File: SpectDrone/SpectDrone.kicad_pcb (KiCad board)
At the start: 2 copper layers, 220.1 x 71.1 mm, 64 parts, among them J1 Camera, J2 GPS, J4 BME280, J5-1 BNO055-1, J5-2 BNO055-2, Q1 FDN340P, Q2 FDN340P, SW1 SW_Push, SW2 SW_Push, SW3 SW_Push, SW4 SW_Push, SW5 SW_Push, SW6 SW_Push, U1 C12666MA, U2 C12666MA, U3 LM7805_TO220, U4 MCP112-300E/TO, U5 MCP112-300E/TO, U6 LM7805_TO220, U7 Teensy3.2

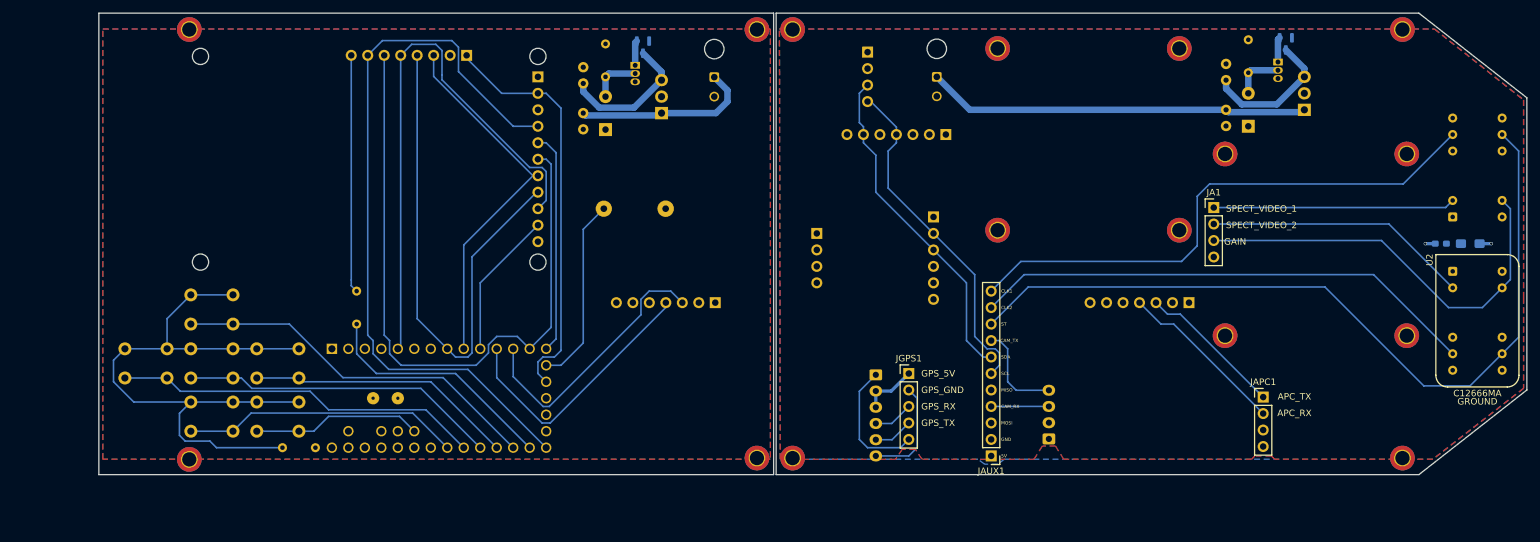
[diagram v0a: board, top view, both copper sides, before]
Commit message: SpectDrone Development
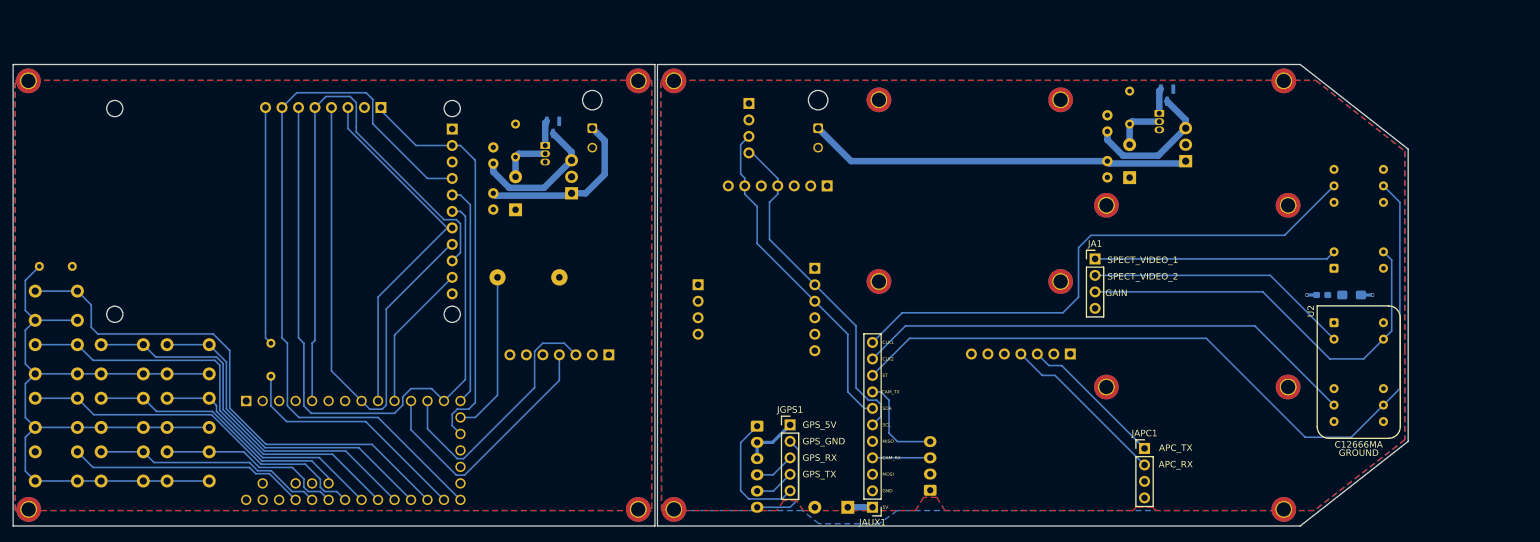
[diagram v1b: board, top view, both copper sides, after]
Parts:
- added D3: Ge, Diode_THT:D_T-1_P5.08mm_Horizontal, B.Cu at (170.9, 142.5)
- added SW0: SW_Push, Button_Switch_THT:SW_PUSH_6mm_H4.3mm, B.Cu at (52.2, 109.2)
- added SW7: SW_Push, Button_Switch_THT:SW_PUSH_6mm_H4.3mm, B.Cu at (72.5, 134.0)
- added SW8: SW_Push, Button_Switch_THT:SW_PUSH_6mm_H4.3mm, B.Cu at (62.4, 134.0)
- added SW9: SW_Push, Button_Switch_THT:SW_PUSH_6mm_H4.3mm, B.Cu at (52.2, 134.0)
- moved RSW1 46.7 mm to (51.4, 105.4)
- moved SW6 34.1 mm to (52.2, 125.7)
- moved H14 26.0 mm to (44.7, 76.8)
- moved H15 25.9 mm to (44.7, 142.9)
- moved SW3 24.0 mm to (52.2, 117.5)
- moved SW2 24.0 mm to (62.4, 117.5)
- moved JBAT2 20.4 mm to (131.6, 84.1)
- moved C1 19.9 mm to (244.0, 109.8)
- moved C2 19.9 mm to (248.6, 109.8)
- moved H1 19.9 mm to (238.1, 142.9)
- moved H13 19.9 mm to (138.7, 76.8)
- moved H16 19.9 mm to (138.7, 142.9)
- moved H2 19.9 mm to (238.1, 76.8)
- moved H3 19.9 mm to (144.2, 76.8)
- moved H4 19.9 mm to (144.2, 142.9)
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- renumbered R4 to RSW1
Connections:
- BT1 pad 2: /GND4 -> /GND2
- C1 pad 2: /GND2 -> /GND1
- C2 pad 2: /GND2 -> /GND1
- C3 pad 1: /GND2 -> /GND1
- C4 pad 2: /GND2 -> /GND1
- C5 pad 1: /GND4 -> /GND2
- C6 pad 2: /GND4 -> /GND2
- J1 pad 2: /GND2 -> /GND1
- J4 pad 3: /GND2 -> /GND1
- J5-1 pad 4: /GND2 -> /GND1
- JAPC-1 pad 7: /GND2 -> /GND1
- JAPC-2 pad 7: /GND4 -> /GND2
- JAUX1 pad 1: /5V3 -> Net-(JAUX1-Pad1)
- JAUX1 pad 2: /GND2 -> /GND1
- JBAT1 pad 2: /GND2 -> /GND1
- JBAT2 pad 2: /GND4 -> /GND2
- JD1 pad 2: /GND4 -> /GND2
- JD2 pad 3: /GND4 -> /GND2
- JIR1 pad 2: /GND2 -> /GND1
- R1 pad 2: /GND2 -> /GND1
- R2 pad 2: /GND4 -> /GND2
- RSW1 pad 1: /5V4 -> /GND2
- RSW1 pad 2: Net-(SW1-Pad1) -> Net-(RSW1-Pad2)
- SW1 pad 1: Net-(SW1-Pad1) -> /SW1
- SW1 pad 2: /SW1 -> Net-(RSW1-Pad2)
- SW2 pad 1: Net-(SW1-Pad1) -> /SW2
- SW2 pad 2: /SW2 -> Net-(RSW1-Pad2)
- SW3 pad 1: Net-(SW1-Pad1) -> /SW3
- SW3 pad 2: /SW3 -> Net-(RSW1-Pad2)
- SW4 pad 1: Net-(SW1-Pad1) -> /SW4
- SW4 pad 2: /SW4 -> Net-(RSW1-Pad2)
- SW5 pad 1: Net-(SW1-Pad1) -> /SW5
- SW5 pad 2: /SW5 -> Net-(RSW1-Pad2)
- SW6 pad 1: Net-(SW1-Pad1) -> /SW6
- SW6 pad 2: /SW6 -> Net-(RSW1-Pad2)
- U1 pad 3: /GND2 -> /GND1
- U1 pad 5: /GND2 -> /GND1
- U2 pad 3: /GND2 -> /GND1
- U2 pad 5: /GND2 -> /GND1
- U3 pad 2: /GND2 -> /GND1
- U4 pad 3: /GND2 -> /GND1
- U5 pad 3: /GND4 -> /GND2
- U6 pad 2: /GND4 -> /GND2
- U7 pad 1: /GND4 -> /GND2
- U7 pad 17: /GND4 -> /GND2
- U7 pad 22: /SW1 -> /SW0
- U7 pad 23: /SW2 -> /SW1
- U7 pad 24: /SW3 -> /SW2
- U7 pad 25: /SW4 -> /SW3
- U7 pad 26: /SW5 -> /SW4
- U7 pad 27: unconnected-(U7-Pad27) -> /SW6
- U7 pad 28: unconnected-(U7-Pad28) -> /SW7
- U7 pad 29: unconnected-(U7-Pad29) -> /SW8
- U7 pad 30: unconnected-(U7-Pad30) -> /SW9
- U7 pad 37: /SW6 -> /SW5
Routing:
- net Net-(RSW1-Pad2): track 0.00 -> 125.3 mm
- net Net-(SW1-Pad1): track 101.3 -> 0.00 mm
- net /SW0: track 0.00 -> 81.0 mm
- net /SW9: track 0.00 -> 36.7 mm
- net /SW8: track 0.00 -> 35.6 mm
- net /SW6: track 26.2 -> 55.0 mm
- net /SW7: track 0.00 -> 28.7 mm
- net /SW4: track 56.7 -> 37.0 mm
- net /SW2: track 41.4 -> 59.3 mm
- net /SW3: track 49.0 -> 66.8 mm
- net /SW1: track 57.6 -> 51.7 mm
- net /VBAT_RTC: track 29.1 -> 25.3 mm
- net Net-(JAUX1-Pad1): track 0.00 -> 3.81 mm
- net /GND1: track 0.00 -> 3.37 mm, vias 0 -> 2
- net /GND2: track 3.37 -> 0.00 mm, vias 2 -> 0
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- added copper zone on F.Cu, net /GND1
- removed copper zone on F.Cu, net /GND4
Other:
- board size 220.1 x 71.1 mm -> 215 x 71.1 mm
